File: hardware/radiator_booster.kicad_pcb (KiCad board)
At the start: 4 copper layers, 58 x 47 mm, 60 parts, among them J301 USB_C_Receptacle_USB2.0, J401 Fan1, J402 Fan2, J403 Fan3, J404 Fan4, J405 Fan5, SW301 RESET, SW302 BOOT, U201 SPX3819M5-L-3-3, U301 USBLC6-2SC6, U302 ESP32-C3FH4, U401 EMC2305-1-AP-TR, Y301 40 MHz

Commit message: Fixed routing at intel pwm fan connectors
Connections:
- net /[3] MCU/LNA_IN renamed /[3] MCU/RF_IN
- net Net-(AE301-A) renamed /[3] MCU/RF_ANT
- J401 pad 2: /[4] Fan Control/PWM1 -> unconnected-(J401-Pin_2-Pad2)
- J401 pad 3: /[4] Fan Control/Tach1 -> unconnected-(J401-Pin_3-Pad3)
- J401 pad 4: +5V -> /[4] Fan Control/PWM1
- J402 pad 2: /[4] Fan Control/PWM2 -> unconnected-(J402-Pin_2-Pad2)
- J402 pad 3: /[4] Fan Control/TACH2 -> unconnected-(J402-Pin_3-Pad3)
- J402 pad 4: +5V -> /[4] Fan Control/PWM2
- J403 pad 2: /[4] Fan Control/PWM3 -> unconnected-(J403-Pin_2-Pad2)
- J403 pad 3: /[4] Fan Control/TACH3 -> unconnected-(J403-Pin_3-Pad3)
- J403 pad 4: +5V -> /[4] Fan Control/PWM3
- J404 pad 2: /[4] Fan Control/PWM4 -> unconnected-(J404-Pin_2-Pad2)
- J404 pad 3: /[4] Fan Control/TACH4 -> unconnected-(J404-Pin_3-Pad3)
- J404 pad 4: +5V -> /[4] Fan Control/PWM4
- J405 pad 2: /[4] Fan Control/PWM5 -> unconnected-(J405-Pin_2-Pad2)
- J405 pad 3: /[4] Fan Control/TACH5 -> unconnected-(J405-Pin_3-Pad3)
- J405 pad 4: +5V -> unconnected-(J405-Pin_4-Pad4)

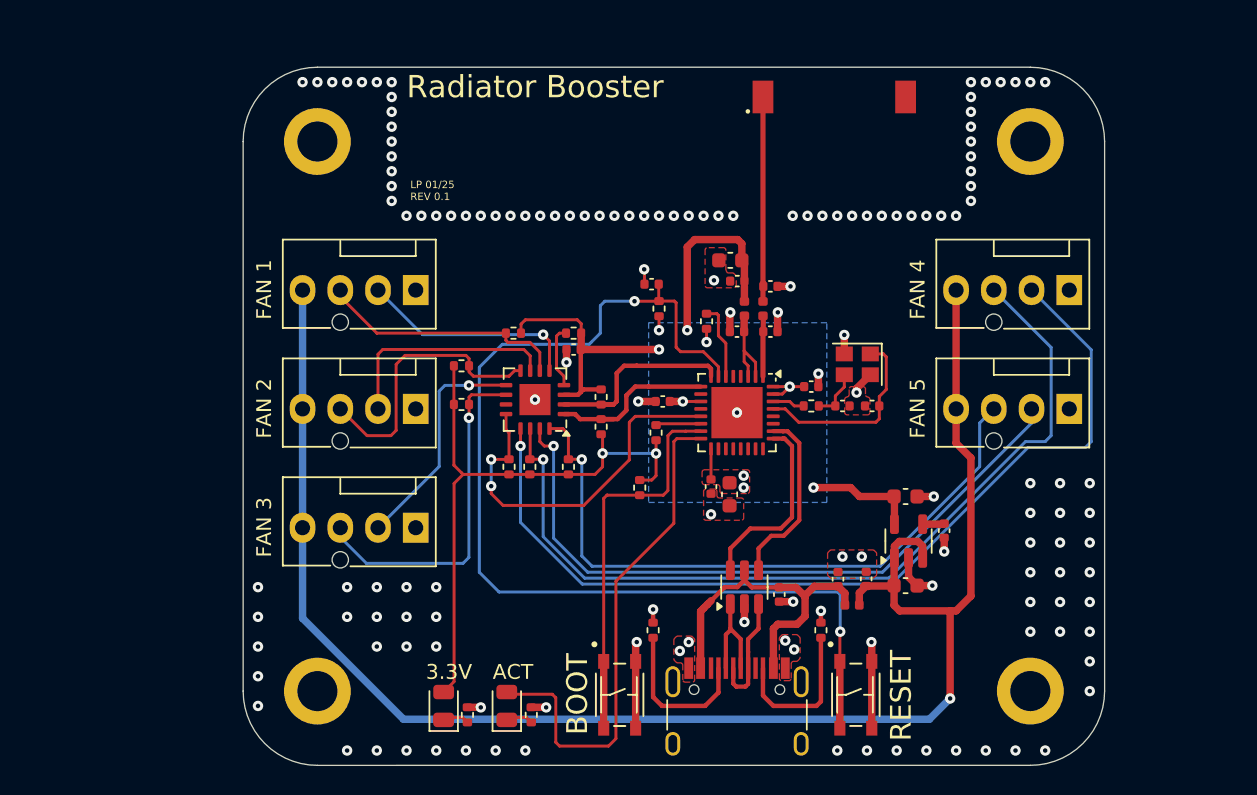
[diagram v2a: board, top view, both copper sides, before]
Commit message: Finished layout for rev 0.2
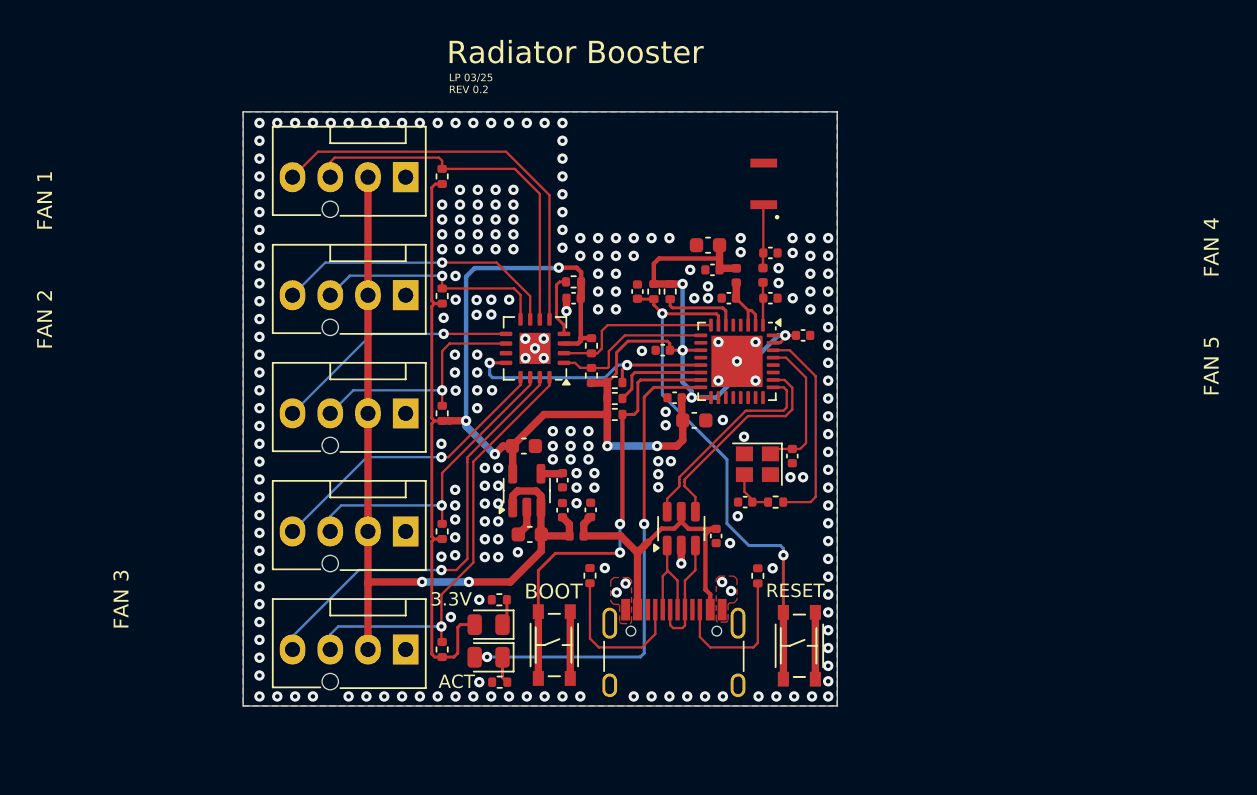
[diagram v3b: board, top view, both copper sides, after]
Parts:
- removed H101, H102, H103, H104: GND, MountingHole:MountingHole_2.7mm_M2.5_ISO14580_Pad
- AE301: value Antenna -> ANT3216LL00R2400A; footprint lzptr:Rainsun-AN9520-245 -> lzptr:ANT3216LL00R2400A
- moved J404 47.5 mm to (147.9, 92.2)
- moved J405 47.5 mm to (147.9, 100.2)
- moved U201 25.9 mm to (156.1, 89.5)
- moved C204 25.9 mm to (158.5, 88.8)
- moved C205 25.9 mm to (155.9, 86.5)
- moved C203 25.5 mm to (156.3, 92.5), turned to 180 degrees
- moved C202 21.0 mm to (158.5, 90.8)
- moved L201 19.1 mm to (159.4, 92.6), turned to 180 degrees
- moved C201 17.3 mm to (160.4, 90.8)
- moved R409 15.0 mm to (150.4, 100.2)
- moved R405 11.6 mm to (150.4, 68.3), turned to 90 degrees
- moved Y301 9.51 mm to (171.6, 87.7)
- moved C303 9.21 mm to (170.8, 90.3), turned to 180 degrees
- moved R401 9.11 mm to (162.0, 82.2), turned to 180 degrees
- moved R201 8.04 mm to (154.2, 96.8), turned to 180 degrees
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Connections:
- J401 pad 2: unconnected-(J401-Pin_2-Pad2) -> +5V
- J401 pad 3: unconnected-(J401-Pin_3-Pad3) -> /[4] Fan Control/TACH1
- J402 pad 2: unconnected-(J402-Pin_2-Pad2) -> +5V
- J402 pad 3: unconnected-(J402-Pin_3-Pad3) -> /[4] Fan Control/TACH2
- J403 pad 2: unconnected-(J403-Pin_2-Pad2) -> +5V
- J403 pad 3: unconnected-(J403-Pin_3-Pad3) -> /[4] Fan Control/TACH3
- J404 pad 2: unconnected-(J404-Pin_2-Pad2) -> +5V
- J404 pad 3: unconnected-(J404-Pin_3-Pad3) -> /[4] Fan Control/TACH4
- J405 pad 2: unconnected-(J405-Pin_2-Pad2) -> +5V
- J405 pad 3: unconnected-(J405-Pin_3-Pad3) -> /[4] Fan Control/TACH5
- J405 pad 4: unconnected-(J405-Pin_4-Pad4) -> /[4] Fan Control/PWM5
- R405 pad 2: /[4] Fan Control/Tach1 -> /[4] Fan Control/TACH1
- U401 pad 6: /[4] Fan Control/Tach1 -> /[4] Fan Control/TACH1
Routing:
- net +5V: track 112.1 -> 54.5 mm, vias 1 -> 2
- net +3.3V: track 89.5 -> 132.4 mm, vias 11 -> 9
- net /[4] Fan Control/PWM4: track 62.3 -> 19.9 mm
- net /[4] Fan Control/TACH4: track 58.9 -> 21.1 mm
- net /[3] MCU/CHIP_EN: track 72.2 -> 36.0 mm
- net /[4] Fan Control/TACH1: track 0.00 -> 25.0 mm
- net GND: track 33.0 -> 13.2 mm, vias 145 -> 251
- net /[4] Fan Control/PWM5: track 46.4 -> 29.1 mm
- net /[4] Fan Control/Tach1: track 17.0 -> 0.00 mm
- net /[4] Fan Control/TACH5: track 44.7 -> 29.6 mm
- net /[4] Fan Control/PWM1: track 15.0 -> 27.6 mm, vias 1 -> 0
- net /[3] MCU/XTAL_P: track 2.18 -> 14.0 mm
- net /[3] MCU/RF_ANT: track 13.8 -> 4.29 mm
- net /FAN_ALERT: track 25.0 -> 17.9 mm
- net /[4] Fan Control/TACH3: track 23.5 -> 16.4 mm
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- added copper zone on B.Cu, net GND
- removed copper zone on B.Cu, net +3.3V
- removed copper zone on F.Cu, net +3.3V
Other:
- board size 58 x 47 mm -> 40 x 40 mm
- board text added: "LP 03/25 REV 0.2"
- board text removed: "LP 01/25 REV 0.1"
